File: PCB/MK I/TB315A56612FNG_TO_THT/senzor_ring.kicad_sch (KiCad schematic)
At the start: 29 parts, among them J1 Conn_01x06_Pin, J3 Conn_01x06_Pin, U1 QRE1113GR, U10 QRE1113GR, U11 QRE1113GR, U12 QRE1113GR, U13 QRE1113GR, U2 QRE1113GR, U3 QRE1113GR, U4 QRE1113GR, U9 QRE1113GR

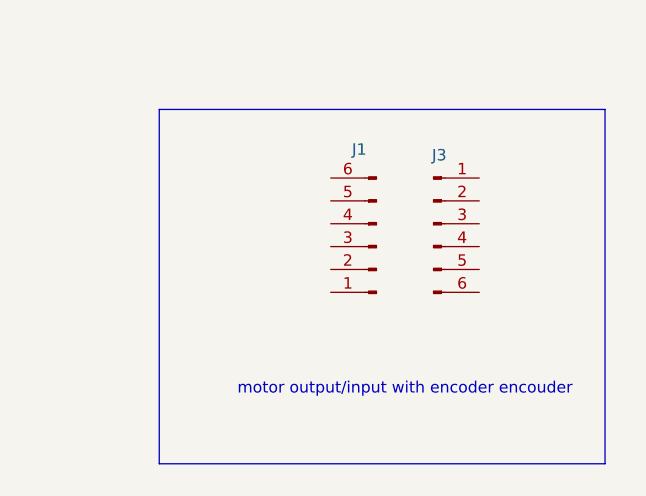
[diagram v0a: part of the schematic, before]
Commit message: saveee
s
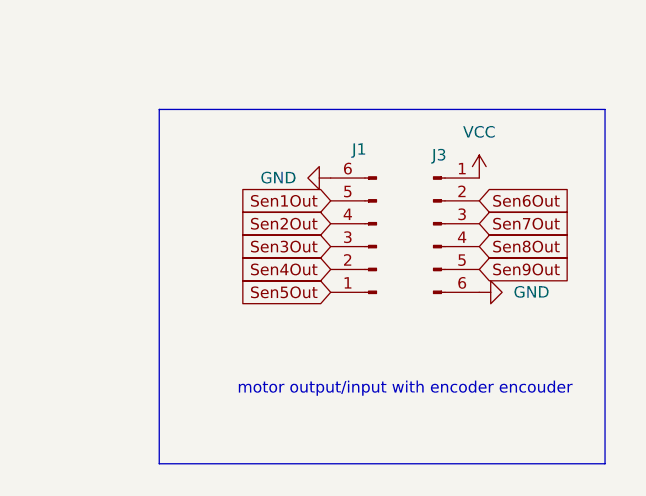
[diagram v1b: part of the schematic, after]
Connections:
- net GND: now also J1.6 (Pin_6), J3.6 (Pin_6)
- net Sen1Out: now also J1.5 (Pin_5)
- net Sen2Out: now also J1.4 (Pin_4)
- net Sen3Out: now also J1.3 (Pin_3)
- net Sen4Out: now also J1.2 (Pin_2)
- net Sen5Out: now also J1.1 (Pin_1)
- net Sen6Out: now also J3.2 (Pin_2)
- net Sen7Out: now also J3.3 (Pin_3)
- net Sen8Out: now also J3.4 (Pin_4)
- net Sen9Out: now also J3.5 (Pin_5)
- net VCC: now also J3.1 (Pin_1)
